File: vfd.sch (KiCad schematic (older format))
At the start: 1 part

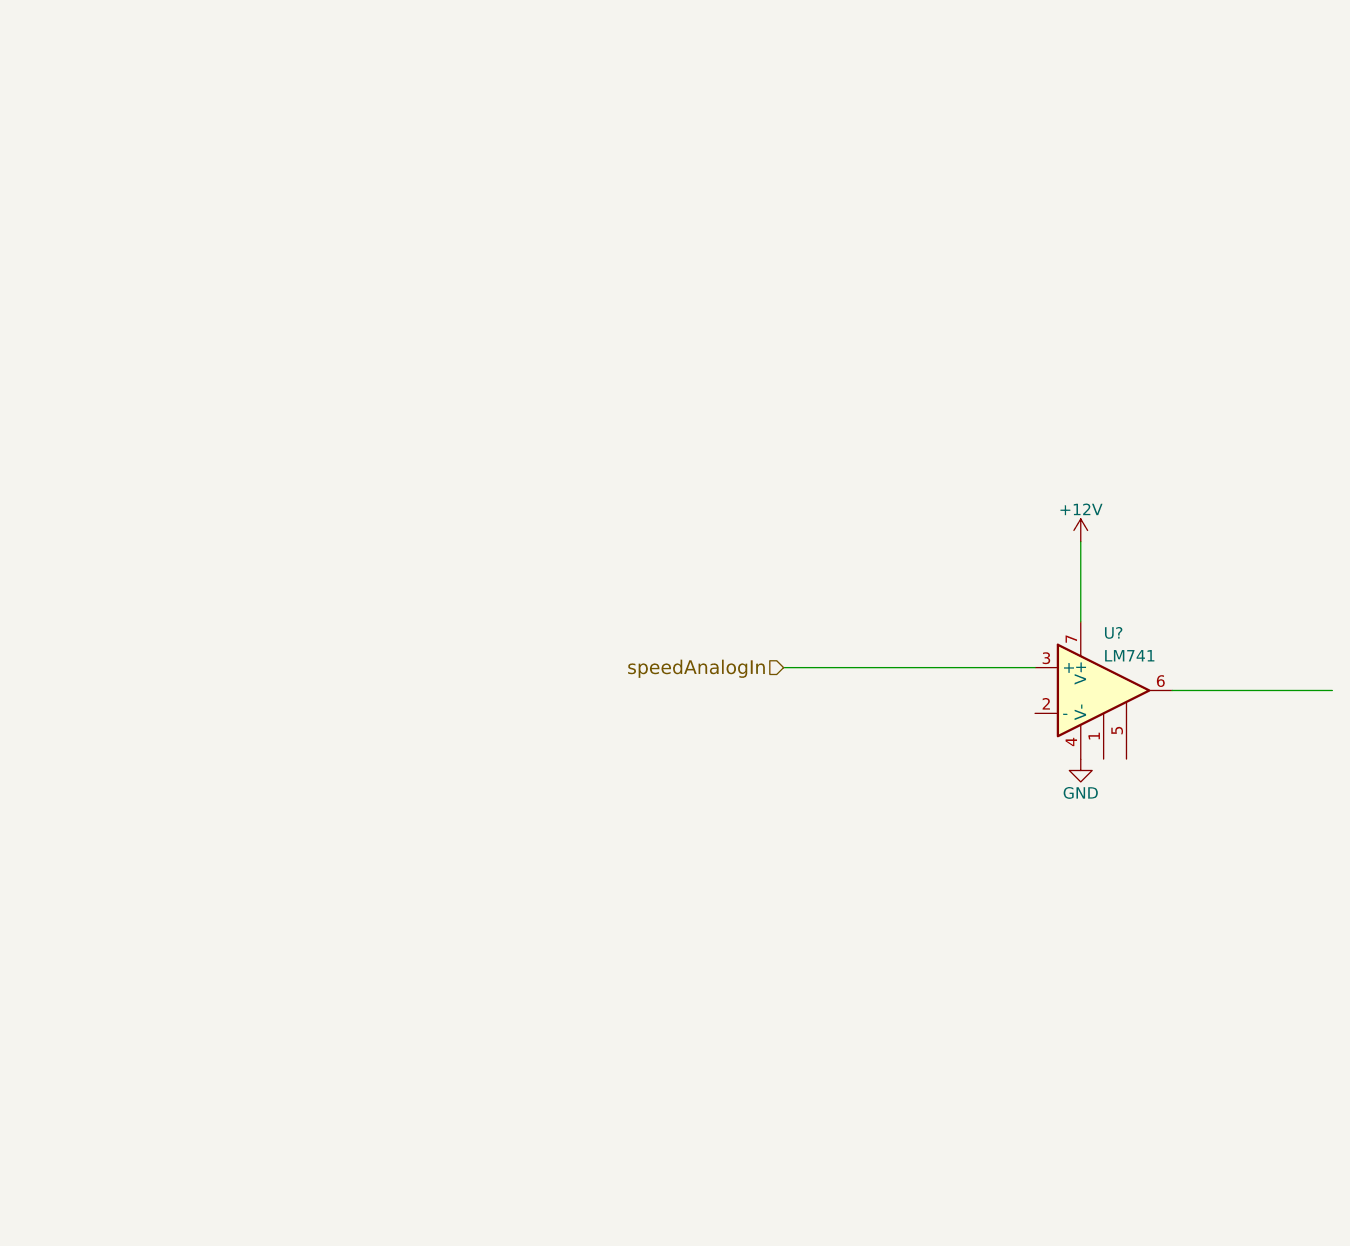
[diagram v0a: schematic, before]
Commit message: Add files via upload
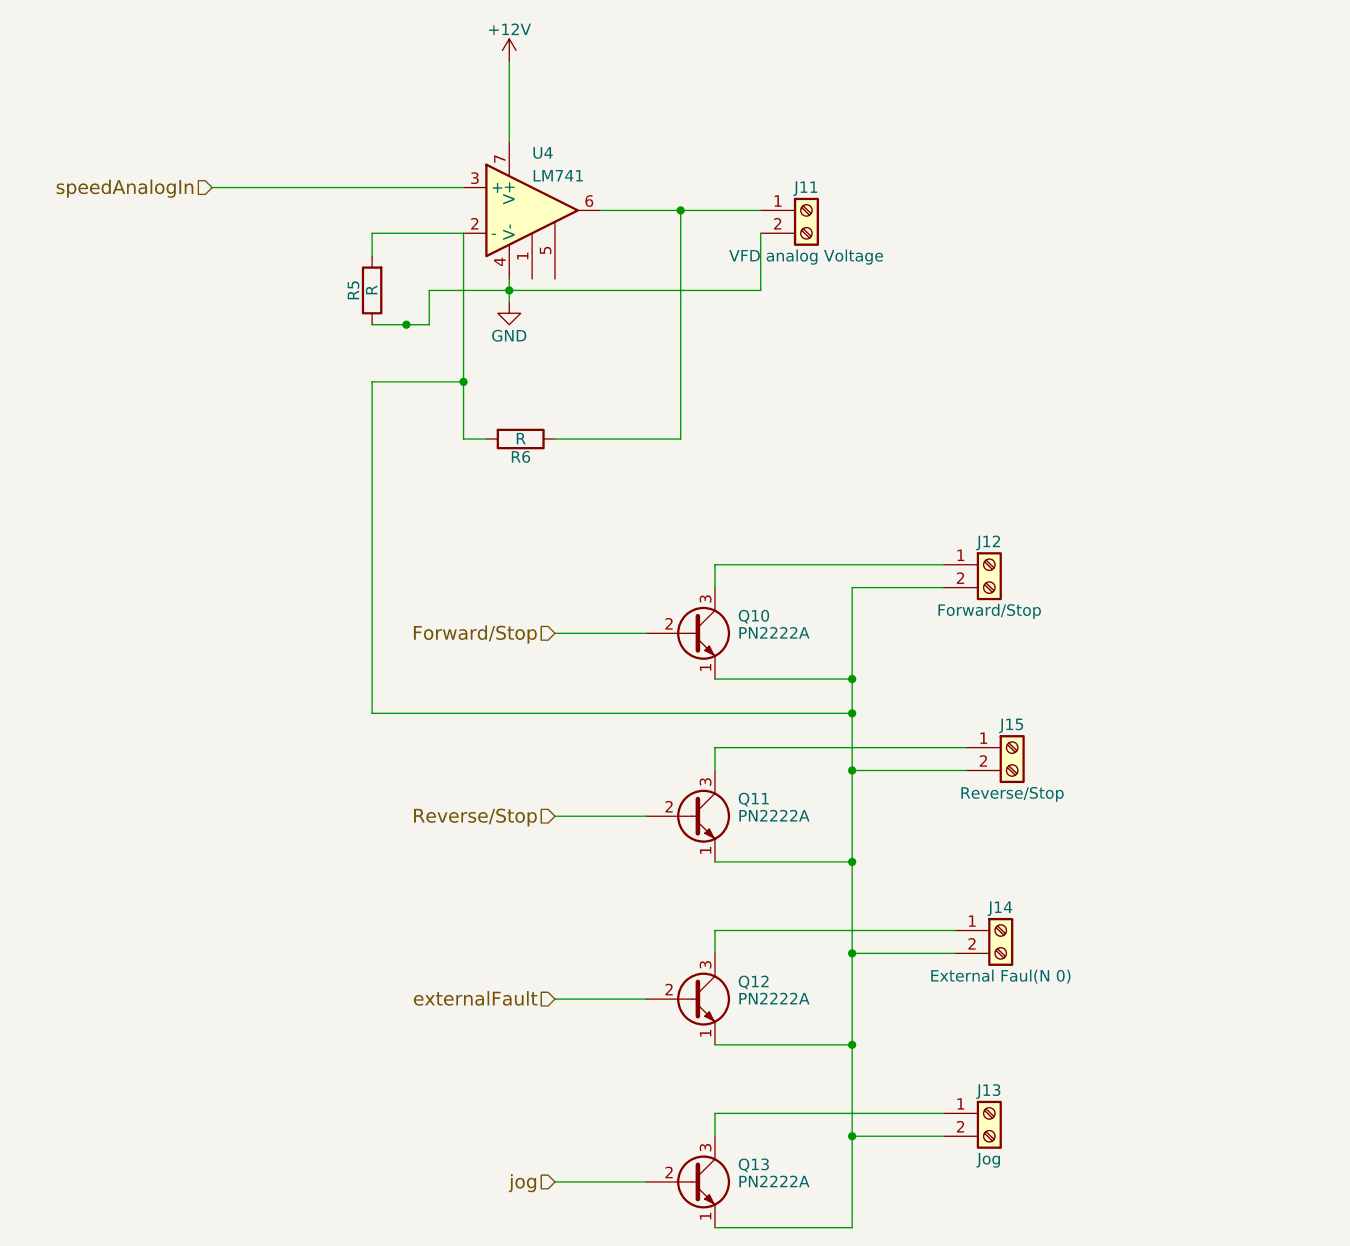
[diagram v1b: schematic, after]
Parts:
- added J11: VFD analog Voltage, symbol Screw_Terminal_01x02
- added J12: Forward/Stop, symbol Screw_Terminal_01x02
- added J13: Jog, symbol Screw_Terminal_01x02
- added J14: External Faul(N 0), symbol Screw_Terminal_01x02
- added J15: Reverse/Stop, symbol Screw_Terminal_01x02
- added Q10, Q11, Q12, Q13: PN2222A, TO_SOT_Packages_THT:TO-92_Molded_Narrow, symbol PN2222A
- added R5, R6: R, symbol R
- gave numbers to parts that had none: 1
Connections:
- net labels added: Forward/Stop, Reverse/Stop, externalFault, jog
- wire segments 3 -> 38
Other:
- moved on the sheet: U4

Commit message: Add files via upload
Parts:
- J11, J12, J13, J14, J15: footprint (none) -> Connectors_Terminal_Blocks:TerminalBlock_Altech_AK300-2_P5.00mm
- R5, R6: footprint (none) -> Resistors_THT:R_Axial_DIN0207_L6.3mm_D2.5mm_P10.16mm_Horizontal
- U4: footprint (none) -> Housings_DIP:DIP-8_W10.16mm_LongPads
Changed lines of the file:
@@
 F 0 "U4" H 3200 2000 50  0000 L CNN
 F 1 "LM741" H 3200 1900 50  0000 L CNN
-F 2 "" H 3250 1800 50  0001 C CNN
+F 2 "Housings_DIP:DIP-8_W10.16mm_LongPads" H 3250 1800 50  0001 C CNN
 F 3 "" H 3350 1900 50  0001 C CNN
 	1    3200 1750
@@
 speedAnalogIn
 $Comp
-L +12V #PWR08
+L +12V #PWR09
 U 1 1 5AC7CE3D
 P 3100 1100
-F 0 "#PWR08" H 3100 950 50  0001 C CNN
+F 0 "#PWR09" H 3100 950 50  0001 C CNN
 F 1 "+12V" H 3100 1240 50  0000 C CNN
 F 2 "" H 3100 1100 50  0001 C CNN
@@
 $EndComp
 $Comp
-L GND #PWR09
+L GND #PWR010
 U 1 1 5AC7CE54
 P 3100 2150
-F 0 "#PWR09" H 3100 1900 50  0001 C CNN
+F 0 "#PWR010" H 3100 1900 50  0001 C CNN
 F 1 "GND" H 3100 2000 50  0000 C CNN
 F 2 "" H 3100 2150 50  0001 C CNN
@@
 F 0 "J11" H 4400 1850 50  0000 C CNN
 F 1 "VFD analog Voltage" H 4400 1550 50  0000 C CNN
-F 2 "" H 4400 1750 50  0001 C CNN
+F 2 "Connectors_Terminal_Blocks:TerminalBlock_Altech_AK300-2_P5.00mm" H 4400 1750 50  0001 C CNN
 F 3 "" H 4400 1750 50  0001 C CNN
 	1    4400 1750
@@
 F 0 "R6" V 3230 2750 50  0000 C CNN
 F 1 "R" V 3150 2750 50  0000 C CNN
-F 2 "" V 3080 2750 50  0001 C CNN
+F 2 "Resistors_THT:R_Axial_DIN0207_L6.3mm_D2.5mm_P10.16mm_Horizontal" V 3080 2750 50  0001 C CNN
 F 3 "" H 3150 2750 50  0001 C CNN
 	1    3150 2750
@@
 F 0 "R5" V 2580 2100 50  0000 C CNN
 F 1 "R" V 2500 2100 50  0000 C CNN
-F 2 "" V 2430 2100 50  0001 C CNN
+F 2 "Resistors_THT:R_Axial_DIN0207_L6.3mm_D2.5mm_P10.16mm_Horizontal" V 2430 2100 50  0001 C CNN
 F 3 "" H 2500 2100 50  0001 C CNN
 	1    2500 2100
@@
 F 0 "J12" H 5200 3400 50  0000 C CNN
 F 1 "Forward/Stop" H 5200 3100 50  0000 C CNN
-F 2 "" H 5200 3300 50  0001 C CNN
+F 2 "Connectors_Terminal_Blocks:TerminalBlock_Altech_AK300-2_P5.00mm" H 5200 3300 50  0001 C CNN
 F 3 "" H 5200 3300 50  0001 C CNN
 	1    5200 3300
@@
 F 0 "J15" H 5300 4200 50  0000 C CNN
 F 1 "Reverse/Stop" H 5300 3900 50  0000 C CNN
-F 2 "" H 5300 4100 50  0001 C CNN
+F 2 "Connectors_Terminal_Blocks:TerminalBlock_Altech_AK300-2_P5.00mm" H 5300 4100 50  0001 C CNN
 F 3 "" H 5300 4100 50  0001 C CNN
 	1    5300 4100
@@
 F 0 "J13" H 5200 5800 50  0000 C CNN
 F 1 "Jog" H 5200 5500 50  0000 C CNN
-F 2 "" H 5200 5700 50  0001 C CNN
+F 2 "Connectors_Terminal_Blocks:TerminalBlock_Altech_AK300-2_P5.00mm" H 5200 5700 50  0001 C CNN
 F 3 "" H 5200 5700 50  0001 C CNN
 	1    5200 5700
@@
 F 0 "J14" H 5250 5000 50  0000 C CNN
 F 1 "External Faul(N 0)" H 5250 4700 50  0000 C CNN
-F 2 "" H 5250 4900 50  0001 C CNN
+F 2 "Connectors_Terminal_Blocks:TerminalBlock_Altech_AK300-2_P5.00mm" H 5250 4900 50  0001 C CNN
 F 3 "" H 5250 4900 50  0001 C CNN
 	1    5250 4900
